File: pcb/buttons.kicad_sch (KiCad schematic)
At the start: 91 parts, among them J3 MSP_SBW, SW1 Off, SW10 R_LCD3, SW11 R_LCD4, SW12 LCD_LEFT, SW13 LCD_RIGHT, SW14 Glow, SW15 Device, SW16 Media, SW17 Mute, SW18 Prev, SW19 Vol+, SW2 Activities, SW20 Vol-, SW21 Ch+, SW22 Ch-, SW23 Dpad_Up, SW24 Dpad_Left, SW25 Dpad_Right, SW26 Dpad_Down, SW27 Dpad_OK, SW28 PgUp, SW29 PgDown, SW3 Help, SW30 Menu, SW31 Exit, SW32 Guide, SW33 Info, SW34 Stop, SW35 Replay, SW36 Skip, SW37 Play, SW38 Rec, SW39 Rew, SW4 L_LCD1, SW40 Fwd, SW41 Pause, SW42 KP_1, SW43 KP_2, SW44 KP_3, SW45 KP_4, SW46 KP_5, SW47 KP_6, SW48 KP_7, SW49 KP_8, SW5 L_LCD2, SW50 KP_9, SW51 KP_0, SW52 KP_Clear, SW53 KP_Enter, SW6 L_LCD3, SW7 L_LCD4, SW8 R_LCD1, SW9 R_LCD2, U1 MSP430G2553IPW28

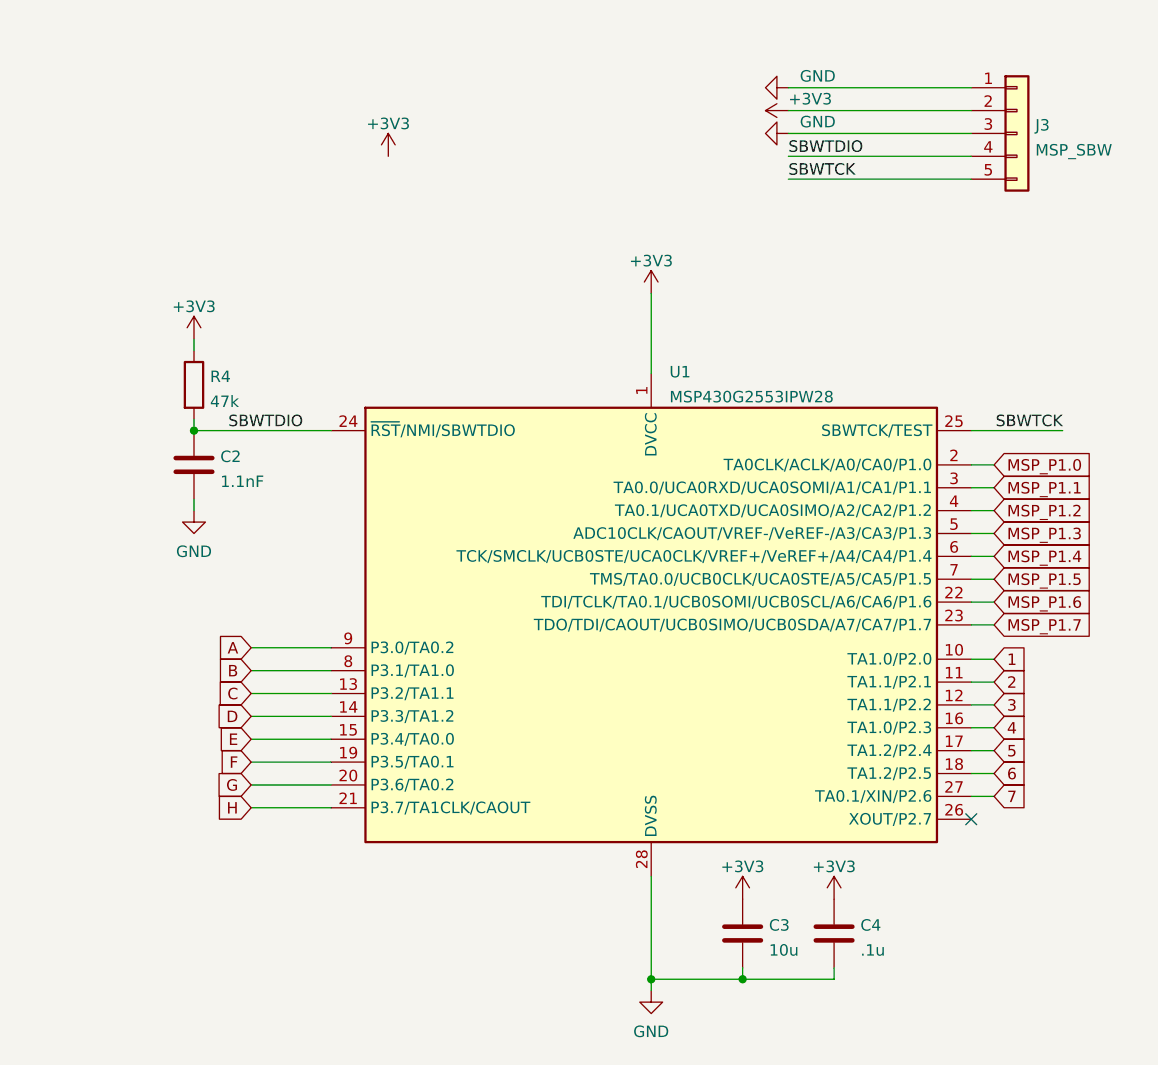
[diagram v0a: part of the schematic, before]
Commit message: alpha2 pcb
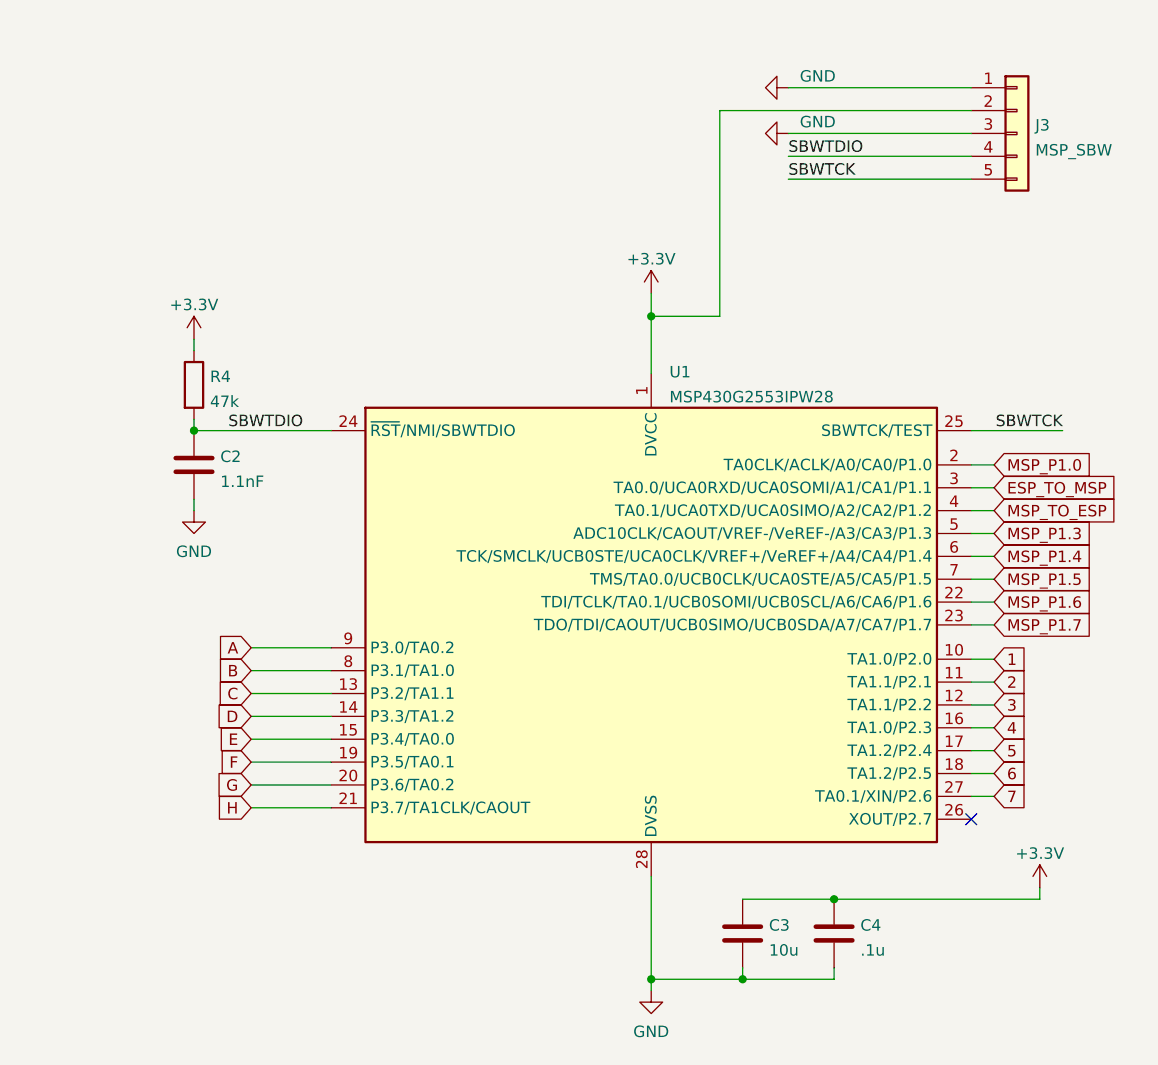
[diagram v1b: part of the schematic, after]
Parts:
- D1, D10, D11, D12, D13, D14, D15, D16, D17, D18, D19, D2, D20, D21, D22, D23, D24, D25, D26, D27, D28, D29, D3, D30, D31, D32, D4, D5, D6, D7, D8, D9: footprint 880+:C265_reverse_mount_led -> 880+:C265_reverse_mount_led_DRC
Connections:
- net +3V3 renamed +3.3V
- net MSP_P1.1 renamed ESP_TO_MSP
- net MSP_P1.2 renamed MSP_TO_ESP

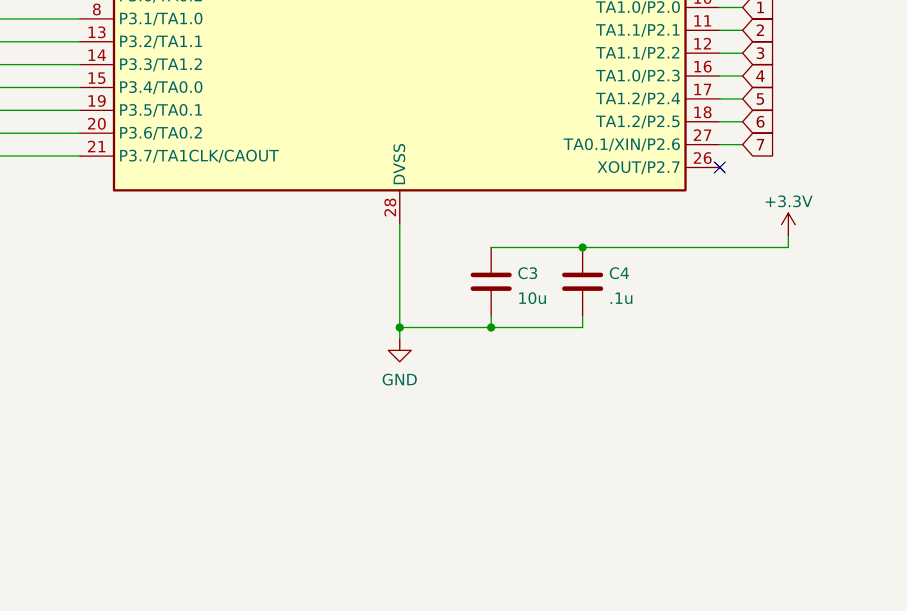
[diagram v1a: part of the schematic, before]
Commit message: current working kikad
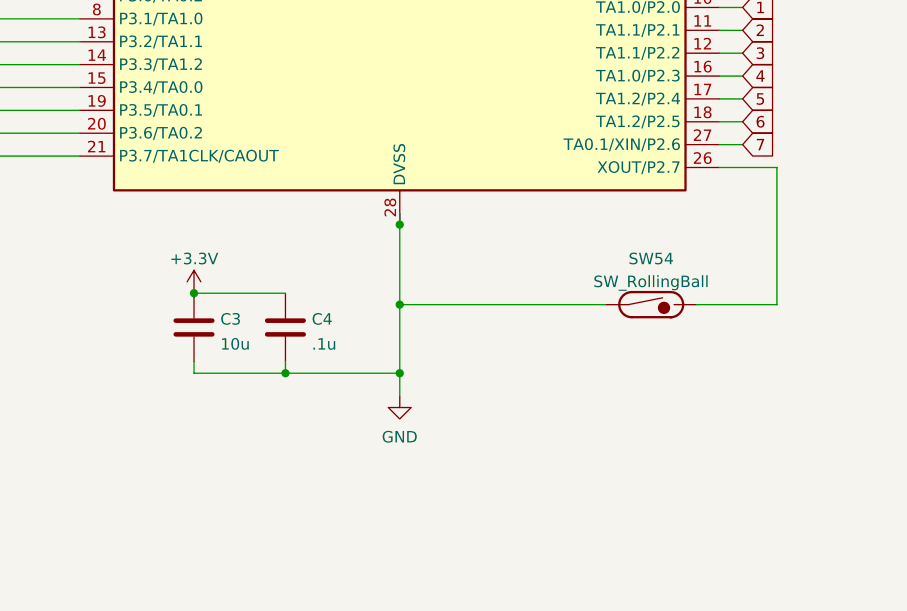
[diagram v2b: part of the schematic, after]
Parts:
- added SW54: SW_RollingBall, Resistor_SMD:R_1210_3225Metric, symbol 880+:SW_RollingBall
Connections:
- net GND: now also SW54.1
- net at U1.26 (XOUT/P2.7): now also SW54.2
- no-connect marks 1 -> 0
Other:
- moved on the sheet: C3, C4
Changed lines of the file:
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@@
   (junction (at 76.2 185.42) (diameter 0) (color 0 0 0 0)
   )
+  (junction (at 205.74 128.27) (diameter 0) (color 0 0 0 0)
+  )
   (junction (at 53.34 185.42) (diameter 0) (color 0 0 0 0)
   )
@@
   (junction (at 46.99 33.02) (diameter 0) (color 0 0 0 0)
   )
+  (junction (at 218.44 120.65) (diameter 0) (color 0 0 0 0)
+  )
   (junction (at 99.06 171.45) (diameter 0) (color 0 0 0 0)
   )
@@
   (junction (at 57.15 55.88) (diameter 0) (color 0 0 0 0)
   )
-  (junction (at 228.6 123.19) (diameter 0) (color 0 0 0 0)
-  )
   (junction (at 53.34 132.08) (diameter 0) (color 0 0 0 0)
   )
@@
   (junction (at 57.15 30.48) (diameter 0) (color 0 0 0 0)
   )
+  (junction (at 195.58 119.38) (diameter 0) (color 0 0 0 0)
+  )
   (junction (at 46.99 45.72) (diameter 0) (color 0 0 0 0)
   )
@@
   (junction (at 80.01 71.12) (diameter 0) (color 0 0 0 0)
   )
-  (junction (at 238.76 114.3) (diameter 0) (color 0 0 0 0)
-  )
   (junction (at 68.58 146.05) (diameter 0) (color 0 0 0 0)
   )
@@
   (junction (at 45.72 132.08) (diameter 0) (color 0 0 0 0)
   )
+  (junction (at 218.44 128.27) (diameter 0) (color 0 0 0 0)
+  )
   (junction (at 45.72 146.05) (diameter 0) (color 0 0 0 0)
   )
@@
   (junction (at 80.01 58.42) (diameter 0) (color 0 0 0 0)
   )
+  (junction (at 218.44 111.76) (diameter 0) (color 0 0 0 0)
+  )
   (junction (at 90.17 43.18) (diameter 0) (color 0 0 0 0)
   )
@@
   (junction (at 40.64 55.88) (diameter 0) (color 0 0 0 0)
   )
-  (junction (at 218.44 123.19) (diameter 0) (color 0 0 0 0)
-  )
   (junction (at 83.82 173.99) (diameter 0) (color 0 0 0 0)
   )
@@
   (junction (at 46.99 96.52) (diameter 0) (color 0 0 0 0)
   )
-  (no_connect (at 254 105.41))
   (wire (pts (xy 254 81.28) (xy 256.54 81.28))
     (stroke (width 0) (type default))
@@
     (stroke (width 0) (type default))
   )
+  (wire (pts (xy 218.44 120.65) (xy 241.3 120.65))
+    (stroke (width 0) (type default))
+  )
   (wire (pts (xy 45.72 157.48) (xy 45.72 154.94))
     (stroke (width 0) (type default))
@@
     (stroke (width 0) (type default))
   )
-  (wire (pts (xy 218.44 123.19) (xy 218.44 124.46))
+  (wire (pts (xy 218.44 128.27) (xy 218.44 130.81))
     (stroke (width 0) (type default))
   )
@@
     (stroke (width 0) (type default))
   )
-  (wire (pts (xy 228.6 123.19) (xy 238.76 123.19))
+  (wire (pts (xy 195.58 128.27) (xy 205.74 128.27))
     (stroke (width 0) (type default))
   )
@@
     (stroke (width 0) (type default))
   )
-  (wire (pts (xy 218.44 111.76) (xy 218.44 123.19))
+  (wire (pts (xy 218.44 110.49) (xy 218.44 111.76))
     (stroke (width 0) (type default))
   )
@@
     (stroke (width 0) (type default))
   )
-  (wire (pts (xy 261.62 113.03) (xy 261.62 114.3))
-    (stroke (width 0) (type default))
-  )
   (wire (pts (xy 83.82 146.05) (xy 83.82 147.32))
     (stroke (width 0) (type default))
@@
     (stroke (width 0) (type default))
   )
+  (wire (pts (xy 218.44 120.65) (xy 218.44 128.27))
+    (stroke (width 0) (type default))
+  )
   (wire (pts (xy 53.34 160.02) (xy 53.34 161.29))
     (stroke (width 0) (type default))
@@
     (stroke (width 0) (type default))
   )
+  (wire (pts (xy 254 105.41) (xy 260.35 105.41))
+    (stroke (width 0) (type default))
+  )
   (wire (pts (xy 80.01 45.72) (xy 96.52 45.72))
     (stroke (width 0) (type default))
@@
     (stroke (width 0) (type default))
   )
-  (wire (pts (xy 218.44 123.19) (xy 228.6 123.19))
+  (wire (pts (xy 205.74 128.27) (xy 218.44 128.27))
     (stroke (width 0) (type default))
   )
@@
     (stroke (width 0) (type default))
   )
-  (wire (pts (xy 228.6 123.19) (xy 228.6 121.92))
+  (wire (pts (xy 195.58 128.27) (xy 195.58 127))
     (stroke (width 0) (type default))
   )
@@
     (stroke (width 0) (type default))
   )
-  (wire (pts (xy 238.76 123.19) (xy 238.76 121.92))
+  (wire (pts (xy 205.74 128.27) (xy 205.74 127))
     (stroke (width 0) (type default))
   )
@@
     (stroke (width 0) (type default))
   )
+  (wire (pts (xy 260.35 105.41) (xy 260.35 120.65))
+    (stroke (width 0) (type default))
+  )
   (wire (pts (xy 90.17 68.58) (xy 90.17 55.88))
     (stroke (width 0) (type default))
@@
     (stroke (width 0) (type default))
   )
+  (wire (pts (xy 260.35 120.65) (xy 251.46 120.65))
+    (stroke (width 0) (type default))
+  )
   (wire (pts (xy 60.96 157.48) (xy 68.58 157.48))
     (stroke (width 0) (type default))
@@
     (stroke (width 0) (type default))
   )
-  (wire (pts (xy 261.62 114.3) (xy 238.76 114.3))
-    (stroke (width 0) (type default))
-  )
   (wire (pts (xy 63.5 96.52) (xy 80.01 96.52))
     (stroke (width 0) (type default))
@@
     (stroke (width 0) (type default))
   )
-  (wire (pts (xy 228.6 114.3) (xy 238.76 114.3))
+  (wire (pts (xy 195.58 119.38) (xy 205.74 119.38))
+    (stroke (width 0) (type default))
+  )
+  (wire (pts (xy 218.44 111.76) (xy 218.44 120.65))
     (stroke (width 0) (type default))
   )
@@
     )
   )
-  (symbol (lib_id "power:GND") (at 218.44 124.46 0) (unit 1)
+  (symbol (lib_id "power:GND") (at 218.44 130.81 0) (unit 1)
     (in_bom yes) (on_board yes) (dnp no) (fields_autoplaced)
-    (property "Reference" "#PWR06" (at 218.44 130.81 0)
+    (property "Reference" "#PWR06" (at 218.44 137.16 0)
       (effects (font (size 1.27 1.27)) hide)
     )
-    (property "Value" "GND" (at 218.44 129.0225 0)
+    (property "Value" "GND" (at 218.44 135.3725 0)
       (effects (font (size 1.27 1.27)))
     )
-    (property "Footprint" "" (at 218.44 124.46 0)
+    (property "Footprint" "" (at 218.44 130.81 0)
       (effects (font (size 1.27 1.27)) hide)
     )
-    (property "Datasheet" "" (at 218.44 124.46 0)
+    (property "Datasheet" "" (at 218.44 130.81 0)
       (effects (font (size 1.27 1.27)) hide)
     )
@@
     )
   )
+  (symbol (lib_id "880+:SW_RollingBall") (at 246.38 120.65 0) (unit 1)
+    (in_bom yes) (on_board yes) (dnp no) (fields_autoplaced)
+    (property "Reference" "SW54" (at 246.38 115.57 0)
+      (effects (font (size 1.27 1.27)))
+    )
+    (property "Value" "SW_RollingBall" (at 246.38 118.11 0)
+      (effects (font (size 1.27 1.27)))
+    )
+    (property "Footprint" "Resistor_SMD:R_1210_3225Metric" (at 246.38 120.65 0)
+      (effects (font (size 1.27 1.27)) hide)
+    )
+    (property "Datasheet" "~" (at 246.38 120.65 0)
+      (effects (font (size 1.27 1.27)) hide)
+    )
+    (pin "1")
+    (pin "2")
+    (instances
+      (project "800+"
+        (path "/e63e39d7-6ac0-4ffd-8aa3-1841a4541b55/ceed2ac1-ff2d-4a48-84e5-5f8d5045fc04"
+          (reference "SW54") (unit 1)
+        )
+      )
+    )
+  )
   (symbol (lib_id "Device:LED") (at 45.72 179.07 90) (unit 1)
     (in_bom yes) (on_board yes) (dnp no) (fields_autoplaced)
@@
     )
   )
-  (symbol (lib_id "power:+3.3V") (at 261.62 113.03 0) (unit 1)
+  (symbol (lib_id "power:+3.3V") (at 195.58 119.38 0) (unit 1)
     (in_bom yes) (on_board yes) (dnp no)
-    (property "Reference" "#PWR019" (at 261.62 116.84 0)
+    (property "Reference" "#PWR019" (at 195.58 123.19 0)
       (effects (font (size 1.27 1.27)) hide)
     )
-    (property "Value" "+3.3V" (at 261.62 109.22 0)
+    (property "Value" "+3.3V" (at 195.58 115.57 0)
       (effects (font (size 1.27 1.27)))
     )
-    (property "Footprint" "" (at 261.62 113.03 0)
+    (property "Footprint" "" (at 195.58 119.38 0)
       (effects (font (size 1.27 1.27)) hide)
     )
-    (property "Datasheet" "" (at 261.62 113.03 0)
+    (property "Datasheet" "" (at 195.58 119.38 0)
       (effects (font (size 1.27 1.27)) hide)
     )
@@
     )
   )
-  (symbol (lib_id "Device:C") (at 228.6 118.11 0) (unit 1)
+  (symbol (lib_id "Device:C") (at 195.58 123.19 0) (unit 1)
     (in_bom yes) (on_board yes) (dnp no) (fields_autoplaced)
-    (property "Reference" "C3" (at 231.521 117.2015 0)
+    (property "Reference" "C3" (at 198.501 122.2815 0)
       (effects (font (size 1.27 1.27)) (justify left))
     )
-    (property "Value" "10u" (at 231.521 119.9766 0)
+    (property "Value" "10u" (at 198.501 125.0566 0)
       (effects (font (size 1.27 1.27)) (justify left))
     )
-    (property "Footprint" "Capacitor_SMD:C_0805_2012Metric" (at 229.5652 121.92 0)
+    (property "Footprint" "Capacitor_SMD:C_0805_2012Metric" (at 196.5452 127 0)
       (effects (font (size 1.27 1.27)) hide)
     )
-    (property "Datasheet" "~" (at 228.6 118.11 0)
+    (property "Datasheet" "~" (at 195.58 123.19 0)
       (effects (font (size 1.27 1.27)) hide)
     )
@@
     )
   )
-  (symbol (lib_id "Device:C") (at 238.76 118.11 0) (unit 1)
+  (symbol (lib_id "Device:C") (at 205.74 123.19 0) (unit 1)
     (in_bom yes) (on_board yes) (dnp no) (fields_autoplaced)
-    (property "Reference" "C4" (at 241.681 117.2015 0)
+    (property "Reference" "C4" (at 208.661 122.2815 0)
       (effects (font (size 1.27 1.27)) (justify left))
     )
-    (property "Value" ".1u" (at 241.681 119.9766 0)
+    (property "Value" ".1u" (at 208.661 125.0566 0)
       (effects (font (size 1.27 1.27)) (justify left))
     )
-    (property "Footprint" "Capacitor_SMD:C_0805_2012Metric" (at 239.7252 121.92 0)
+    (property "Footprint" "Capacitor_SMD:C_0805_2012Metric" (at 206.7052 127 0)
       (effects (font (size 1.27 1.27)) hide)
     )
-    (property "Datasheet" "~" (at 238.76 118.11 0)
+    (property "Datasheet" "~" (at 205.74 123.19 0)
       (effects (font (size 1.27 1.27)) hide)
     )
